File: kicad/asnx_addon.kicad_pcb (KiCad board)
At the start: 2 copper layers, 61.5 x 43.4 mm, 10 parts, among them J1 OWI1, J2 OWI2, J4 TWI1, J5 TWI2, J7 COM/GPIO, J8 ADC/GPIO

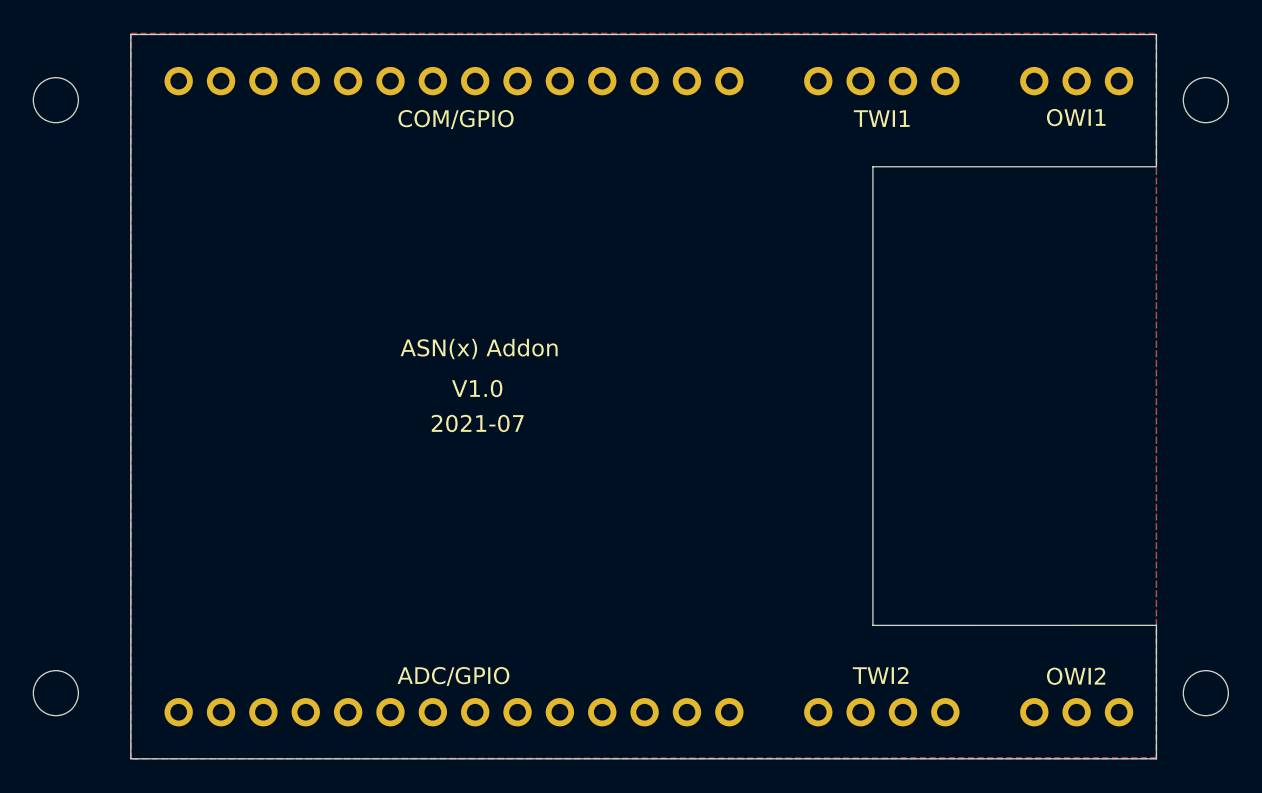
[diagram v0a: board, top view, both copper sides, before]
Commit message: Added initial PCB design (incl. BOM)
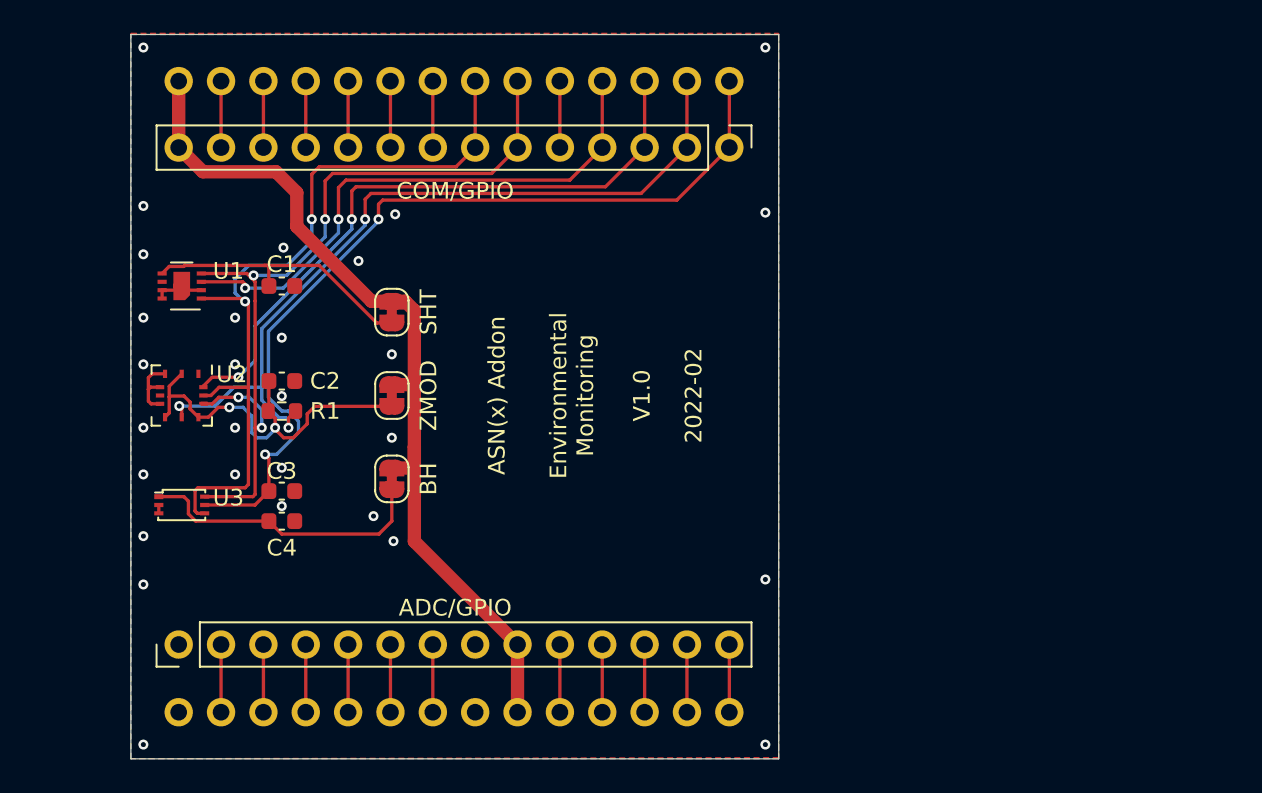
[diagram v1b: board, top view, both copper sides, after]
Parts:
- removed H1, H2, H3, H4: MountingHole, MountingHole:MountingHole_2.7mm_M2.5
- removed the J1 at (175.0, 86.6)
- removed J5: TWI2, Connector_PinHeader_2.54mm:PinHeader_1x04_P2.54mm_Vertical
- added C1: 100n, Capacitor_SMD:C_0603_1608Metric, F.Cu at (124.8, 98.9)
- added C2: 100n, Capacitor_SMD:C_0603_1608Metric, F.Cu at (124.8, 104.6)
- added C3: 100n, Capacitor_SMD:C_0603_1608Metric, F.Cu at (124.8, 111.2)
- added C4: 100n, Capacitor_SMD:C_0603_1608Metric, F.Cu at (124.8, 113.0)
- added JP1: EN_SHT, Jumper:SolderJumper-2_P1.3mm_Bridged_RoundedPad1.0x1.5mm, F.Cu at (131.4, 100.5)
- added JP2: EN_ZMOD, Jumper:SolderJumper-2_P1.3mm_Bridged_RoundedPad1.0x1.5mm, F.Cu at (131.4, 105.5)
- added JP3: EN_BH, Jumper:SolderJumper-2_P1.3mm_Bridged_RoundedPad1.0x1.5mm, F.Cu at (131.4, 110.5)
- added R1: 4k7, Resistor_SMD:R_0603_1608Metric, F.Cu at (124.8, 106.4)
- added U1: SHT30-DIS, my_footprints:Sensirion_DFN-8-1EP_2.5x2.5mm_P0.5mm_EP1.1x1.7mm, F.Cu at (118.8, 98.9)
- added U2: ZMOD4410, my_footprints:ZMOD4410-12-LGA, F.Cu at (118.8, 105.5)
- added U3: BH1750FVI, my_footprints:BH1750FVI-WSOF6I, F.Cu at (118.8, 112.0)
- J2: value OWI2 -> COM/GPIO; footprint Connector_PinHeader_2.54mm:PinHeader_1x03_P2.54mm_Vertical -> Connector_PinHeader_2.54mm:PinHeader_1x14_P2.54mm_Vertical; moved to F.Cu
- J4: value TWI1 -> ADC/GPIO; footprint Connector_PinHeader_2.54mm:PinHeader_1x04_P2.54mm_Vertical -> Connector_PinHeader_2.54mm:PinHeader_1x14_P2.54mm_Vertical; moved to F.Cu
- moved J4 57.1 mm to (118.6, 120.4)
- moved J2 41.1 mm to (151.6, 90.6), turned to 270 degrees
- renumbered J7 to J1, J8 to J3
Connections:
- J1 pad 1: (no net) -> /PC5
- J1 pad 10: (no net) -> /SPI_MOSI
- J1 pad 11: (no net) -> /RXD1
- J1 pad 12: (no net) -> /TXD1
- J1 pad 13: (no net) -> /RESET
- J1 pad 2: (no net) -> /PC4
- J1 pad 3: (no net) -> /PC3
- J1 pad 4: (no net) -> /PC2
- J1 pad 8: (no net) -> /SPI_SCK
- J1 pad 9: (no net) -> /SPI_MISO
- J2 pad 1: +3V3 -> /PC5
- J2 pad 2: GND -> /PC4
- J2 pad 3: (no net) -> /PC3
- J3 pad 10: (no net) -> /PB0
- J3 pad 11: (no net) -> /PB1
- J3 pad 12: (no net) -> /PB2
- J3 pad 13: (no net) -> /PB3
- J3 pad 14: (no net) -> /PB4
- J3 pad 2: (no net) -> /ADC7
- J3 pad 3: (no net) -> /ADC6
- J3 pad 4: (no net) -> /ADC5
- J3 pad 5: (no net) -> /ADC4
- J3 pad 6: (no net) -> /ADC3
- J3 pad 7: (no net) -> /ADC2
- J4 pad 1: +3V3 -> GND
- J4 pad 2: GND -> /ADC7
- J4 pad 3: /I2C_SDA -> /ADC6
- J4 pad 4: /I2C_SCL -> /ADC5
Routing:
- net +3V3: track 0.69 -> 54.0 mm
- net /PC5: track 0.00 -> 52.9 mm, vias 0 -> 2
- net /I2C_SCL: track 0.00 -> 49.8 mm, vias 0 -> 4
- net /PC4: track 0.00 -> 49.1 mm, vias 0 -> 3
- net /I2C_SDA: track 0.00 -> 47.7 mm, vias 0 -> 2
- net /PC3: track 0.00 -> 39.0 mm, vias 0 -> 2
- net /PC2: track 0.00 -> 33.4 mm, vias 0 -> 2
- net /ZMOD_PWR: track 0.00 -> 23.4 mm, vias 0 -> 2
- net /BH_PWR: track 0.00 -> 17.6 mm
- net /SHT_PWR: track 0.00 -> 16.9 mm
- net GND: track 0.00 -> 11.6 mm, vias 0 -> 29
- net /SPI_SCK: track 0.00 -> 4.17 mm
- net /SPI_MISO: track 0.00 -> 4.17 mm
- net /PB0: track 0.00 -> 4.08 mm
- net /PB4: track 0.00 -> 4.06 mm
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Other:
- board size 61.5 x 43.4 mm -> 38.8 x 43.4 mm
- board text added: "2022-02"
- board text added: "BH"
- board text added: "Environmental Monitoring"
- board text added: "SHT"
- board text added: "ZMOD"
- board text removed: "2021-07"
- board text removed: "OWI1"
- board text removed: "OWI2"
- board text removed: "TWI1"
- board text removed: "TWI2"
